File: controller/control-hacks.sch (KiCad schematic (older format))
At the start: 27 parts, among them K18 RELAY_SEPARATED, K19 RELAY_SEPARATED, K20 RELAY_SEPARATED, K21 RELAY_SEPARATED, K22 RELAY_SEPARATED, K23 RELAY_SEPARATED, K24 RELAY_SEPARATED, K25 RELAY_SEPARATED, K26 RELAY_SEPARATED

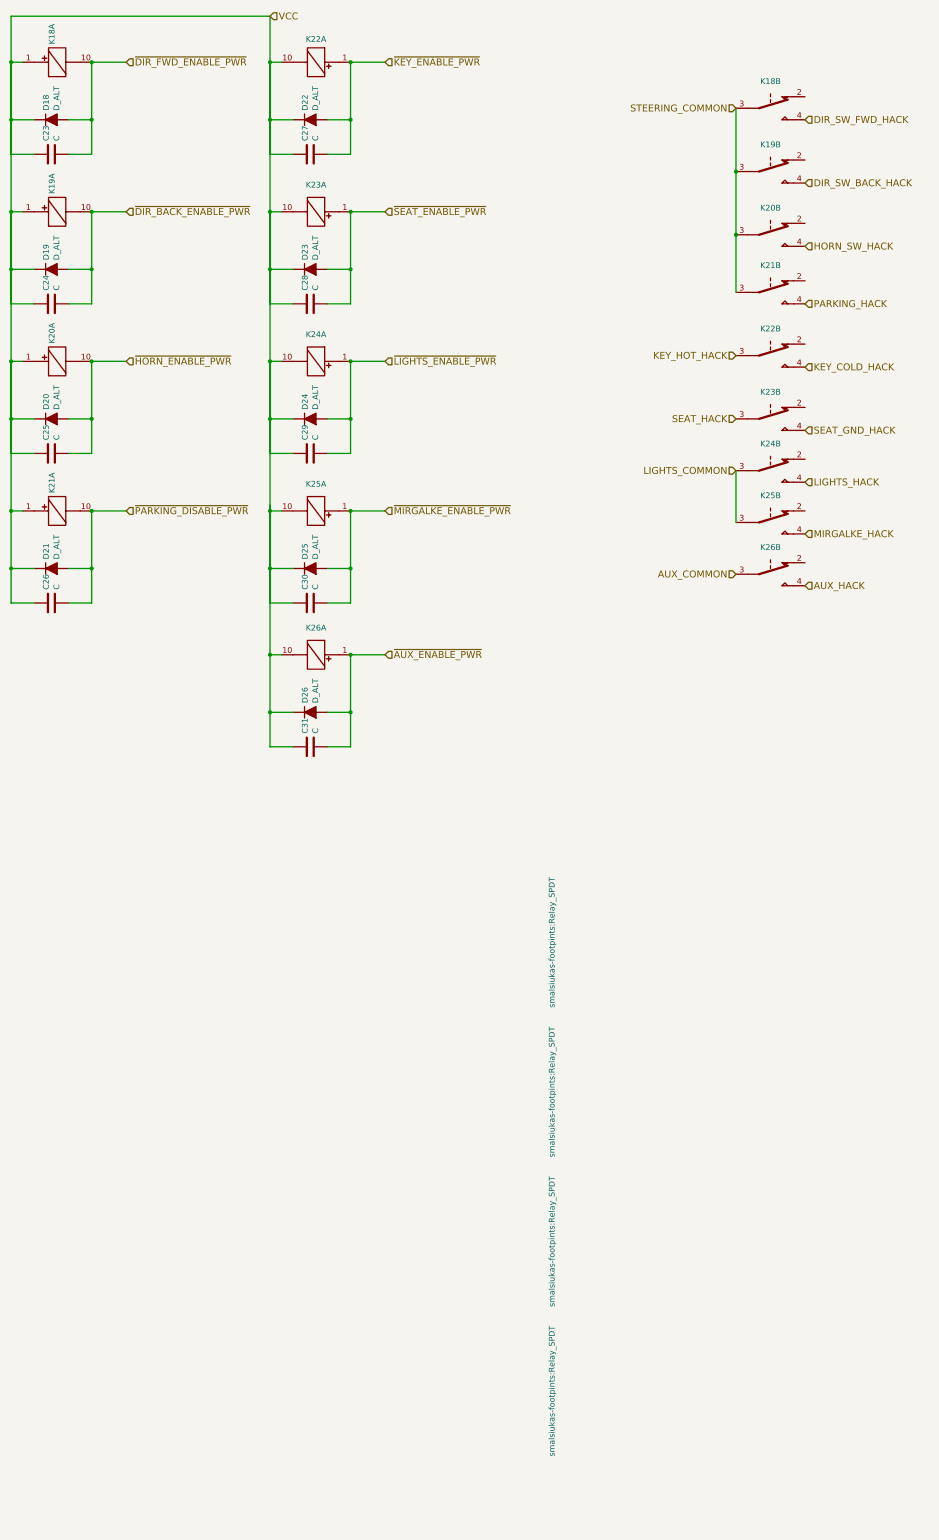
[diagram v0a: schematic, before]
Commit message: More or less final controller board
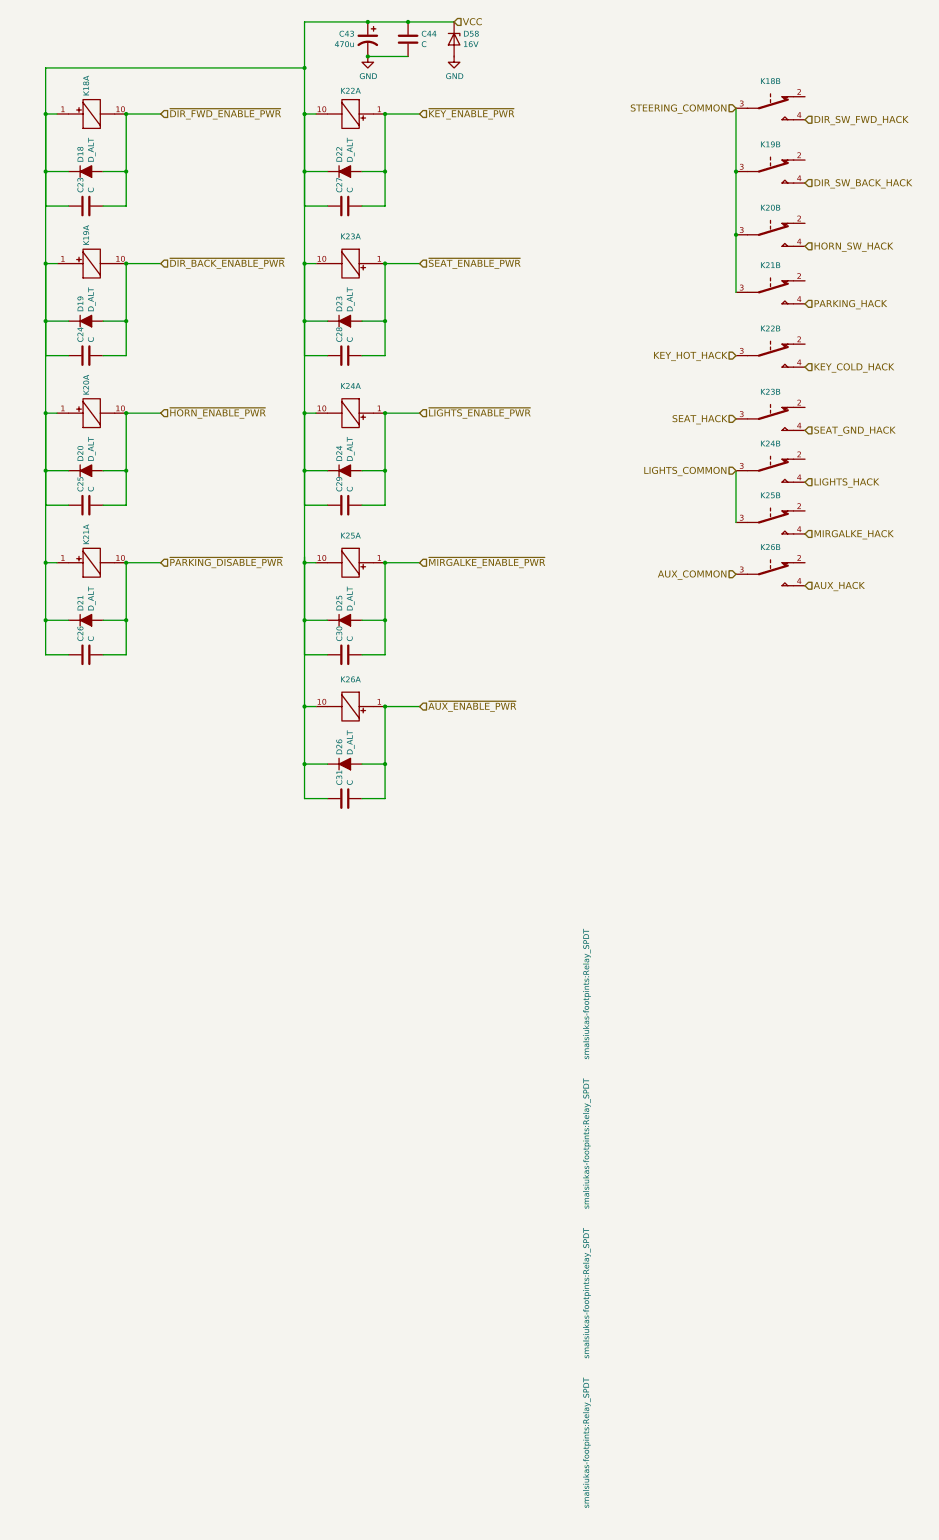
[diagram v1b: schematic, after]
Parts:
- added C43: 470u, Capacitors_ThroughHole:CP_Radial_D16.0mm_P7.50mm, symbol CP1
- added C44: C, Capacitors_SMD:C_1210_HandSoldering, symbol C
- added D58: 16V, Diodes_SMD:D_SMB_Handsoldering, symbol D_Zener
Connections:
- net VCC: now also C43.1, C44.2, D58.1 (K)
- new net GND: C43.2, C44.1, D58.2 (A)
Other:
- moved on the sheet: C23, C24, C25, C26, C27, C28, C29, C30, C31, D18, D19, D20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
